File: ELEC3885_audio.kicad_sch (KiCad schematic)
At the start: 27 parts, among them U2 SGTL5000XNLA3, U3 AP7313

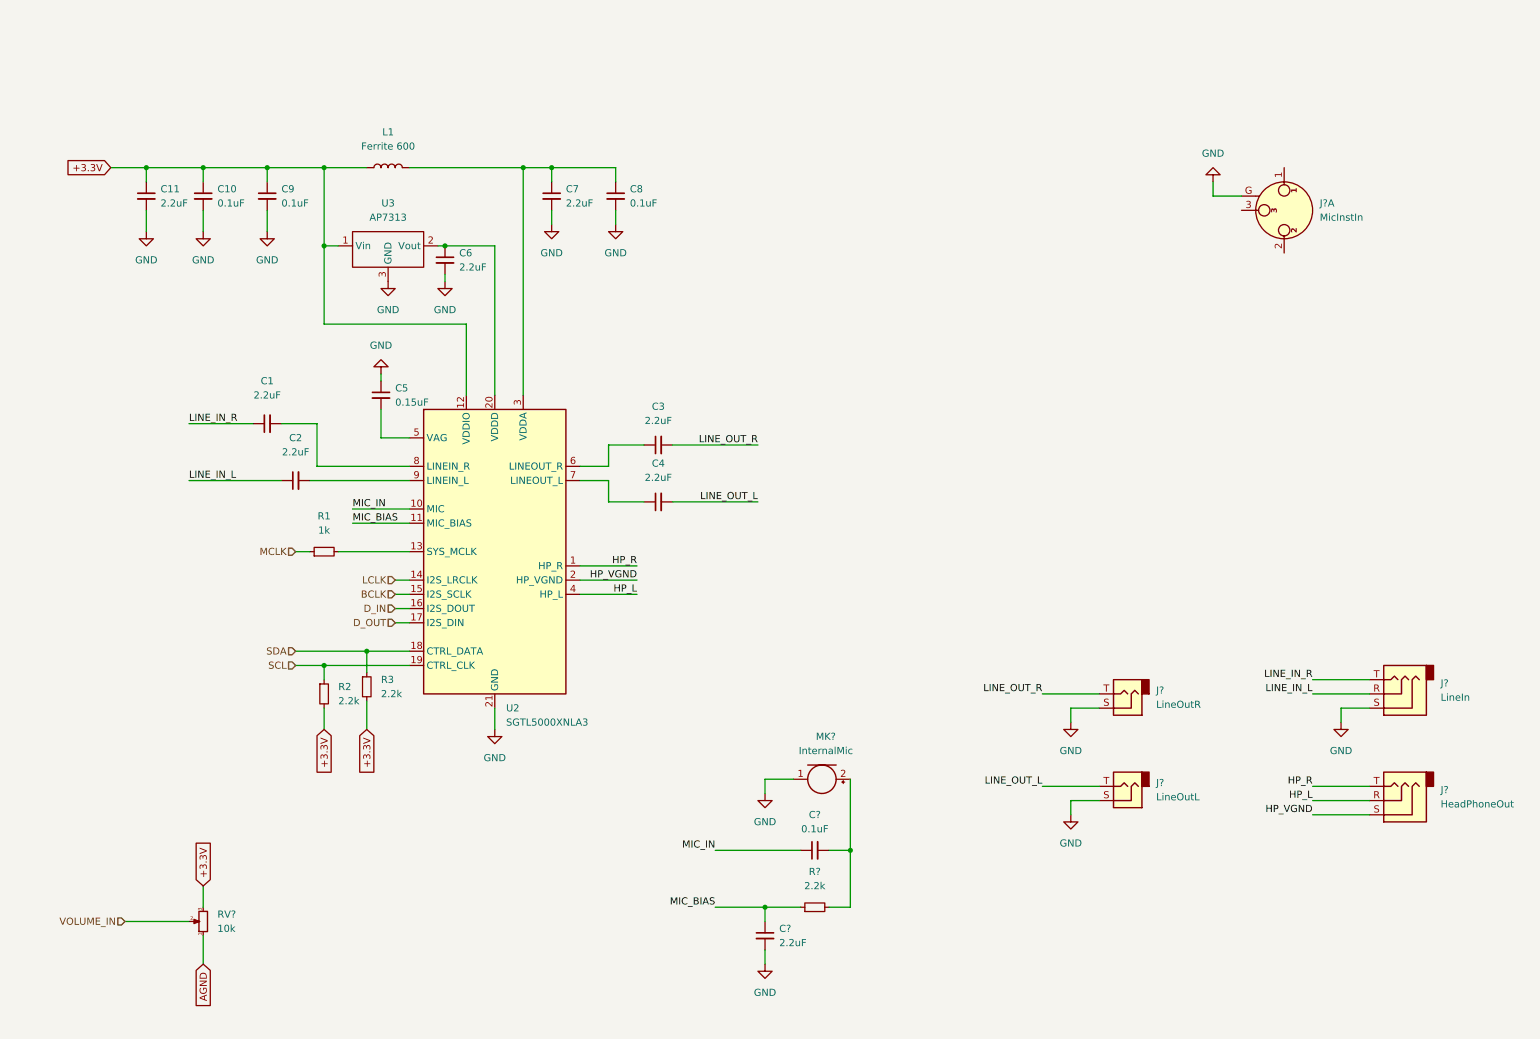
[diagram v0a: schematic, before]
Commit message: Schematic work
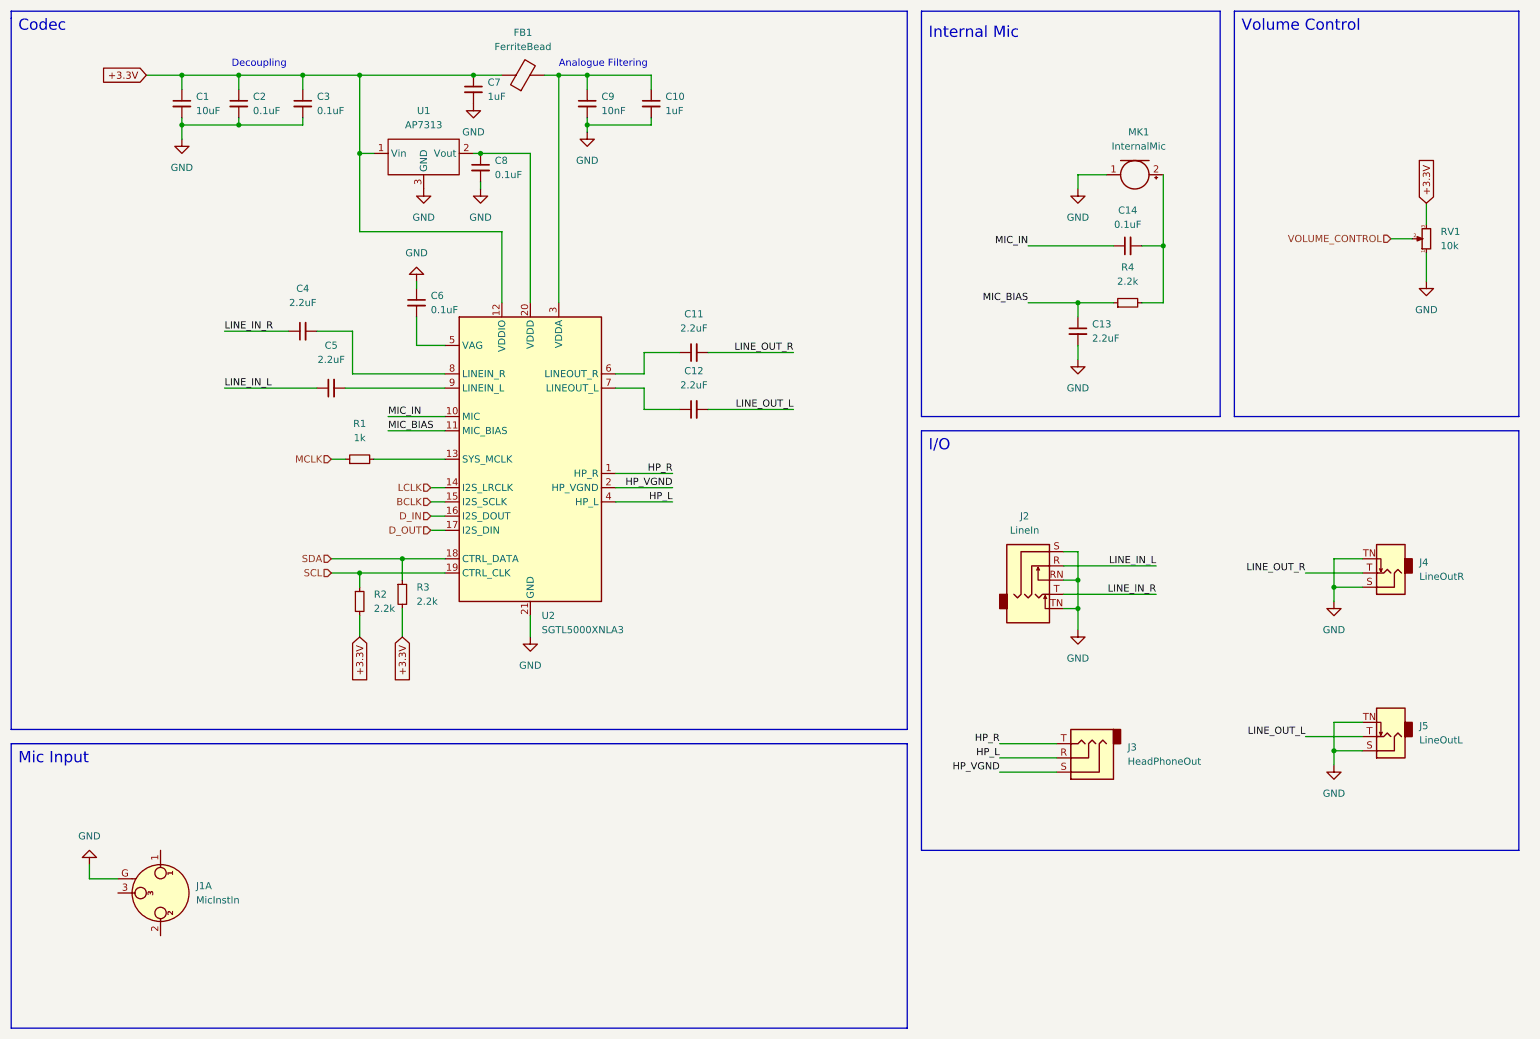
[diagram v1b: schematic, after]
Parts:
- removed J?: LineOutL, symbol Connector:AudioJack2
- removed J?: LineOutR, symbol Connector:AudioJack2
- removed J?: LineIn, symbol Connector:AudioJack3
- removed L1: Ferrite 600, symbol Device:L
- added C7: 1uF, Capacitor_SMD:C_0402_1005Metric, symbol Device:C_Small
- added FB1: FerriteBead, Inductor_SMD:L_0603_1608Metric, symbol Device:FerriteBead
- added J2: LineIn, Connector_Audio:Jack_3.5mm_CUI_SJ1-3535NG_Horizontal, symbol Connector:AudioJack3_SwitchTR
- added J4: LineOutR, Connector_Audio:Jack_6.35mm_Neutrik_NMJ4HCD2_Horizontal, symbol Connector:AudioJack2_SwitchT
- added J5: LineOutL, Connector_Audio:Jack_6.35mm_Neutrik_NMJ4HCD2_Horizontal, symbol Connector:AudioJack2_SwitchT
- C1: renamed from C11; value 2.2uF -> 10uF; footprint (none) -> Capacitor_SMD:C_0603_1608Metric
- C10: renamed from C8; value 0.1uF -> 1uF; footprint (none) -> Capacitor_SMD:C_0402_1005Metric
- C11: renamed from C3; footprint (none) -> Capacitor_SMD:C_0603_1608Metric
- C12: renamed from C4; footprint (none) -> Capacitor_SMD:C_0603_1608Metric
- C13: renamed from C?; footprint (none) -> Capacitor_SMD:C_0603_1608Metric
- C14: renamed from C?; footprint (none) -> Capacitor_SMD:C_0402_1005Metric
- C2: renamed from C10; footprint (none) -> Capacitor_SMD:C_0402_1005Metric
- C3: renamed from C9; footprint (none) -> Capacitor_SMD:C_0402_1005Metric
- C4: renamed from C1; footprint (none) -> Capacitor_SMD:C_0603_1608Metric
- C5: renamed from C2; footprint (none) -> Capacitor_SMD:C_0603_1608Metric
- C6: renamed from C5; value 0.15uF -> 0.1uF; footprint (none) -> Capacitor_SMD:C_0402_1005Metric
- C8: renamed from C6; value 2.2uF -> 0.1uF; footprint (none) -> Capacitor_SMD:C_0402_1005Metric
- C9: renamed from C7; value 2.2uF -> 10nF; footprint (none) -> Capacitor_SMD:C_0402_1005Metric
- J1: renamed from J?; footprint (none) -> Connector_Audio:Jack_XLR_Neutrik_NC3FAAH-0_Horizontal
- J3: renamed from J?; footprint (none) -> Connector_Audio:Jack_3.5mm_CUI_SJ-3523-SMT_Horizontal
- MK1: renamed from MK?; footprint (none) -> Connector_PinSocket_2.54mm:PinSocket_1x02_P2.54mm_Vertical
- R1, R2, R3: footprint (none) -> Resistor_SMD:R_0402_1005Metric
- R4: renamed from R?; footprint (none) -> Resistor_SMD:R_0402_1005Metric
- RV1: renamed from RV?; footprint (none) -> Potentiometer_THT:Potentiometer_Alpha_RD901F-40-00D_Single_Vertical
- U1: renamed from U3; footprint (none) -> LukeLibrary:SOT23
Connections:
- net AGND is gone; now on net GND: RV1.1
- net +3.3V: now also C7.1, FB1.1
- net GND: now also C7.2, J2.RN, J2.S, J2.TN, J4.S, J4.TN, J5.S, J5.TN
- net LINE_IN_L: now also J2.R
- net LINE_IN_R: now also J2.T
- net LINE_OUT_L: now also J5.T
- net LINE_OUT_R: now also J4.T
- net at C10.1, C9.1, U2.3 (VDDA): now also FB1.2
- net VOLUME_IN renamed VOLUME_CONTROL
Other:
- note added: "Analogue Filtering"
- note added: "Codec"
- note added: "Decoupling"
- note added: "I/O"
- note added: "Internal Mic"
- note added: "Mic Input"
- note added: "Volume Control"
- moved on the sheet: C1, C10, C11, C12, C13, C14, C2, C3, C4, C5, C6, C8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
